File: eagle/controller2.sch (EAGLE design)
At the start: 15 parts, among them K1 SRD-05VDC-SL-C, K2 SRD-05VDC-SL-C, T1 BC547, T2 BC547, X1 VCC, X2 IN1, X3 IN2

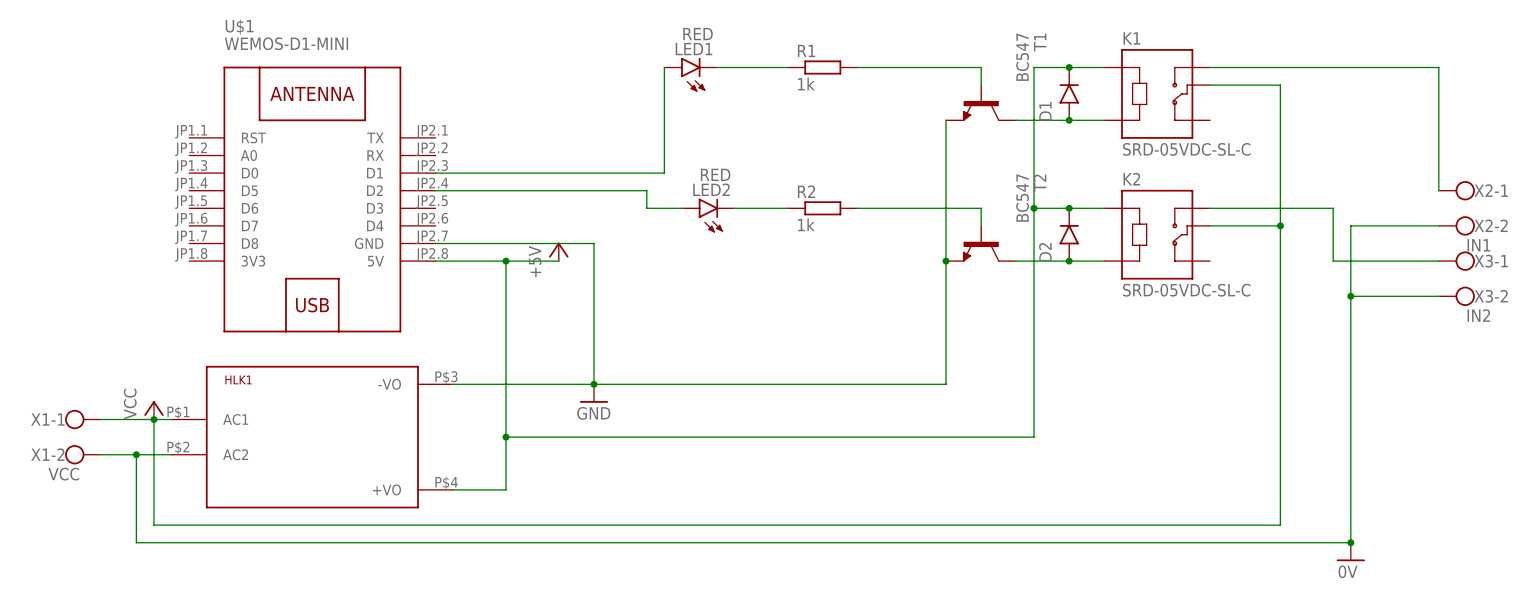
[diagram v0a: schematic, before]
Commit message: refactoring
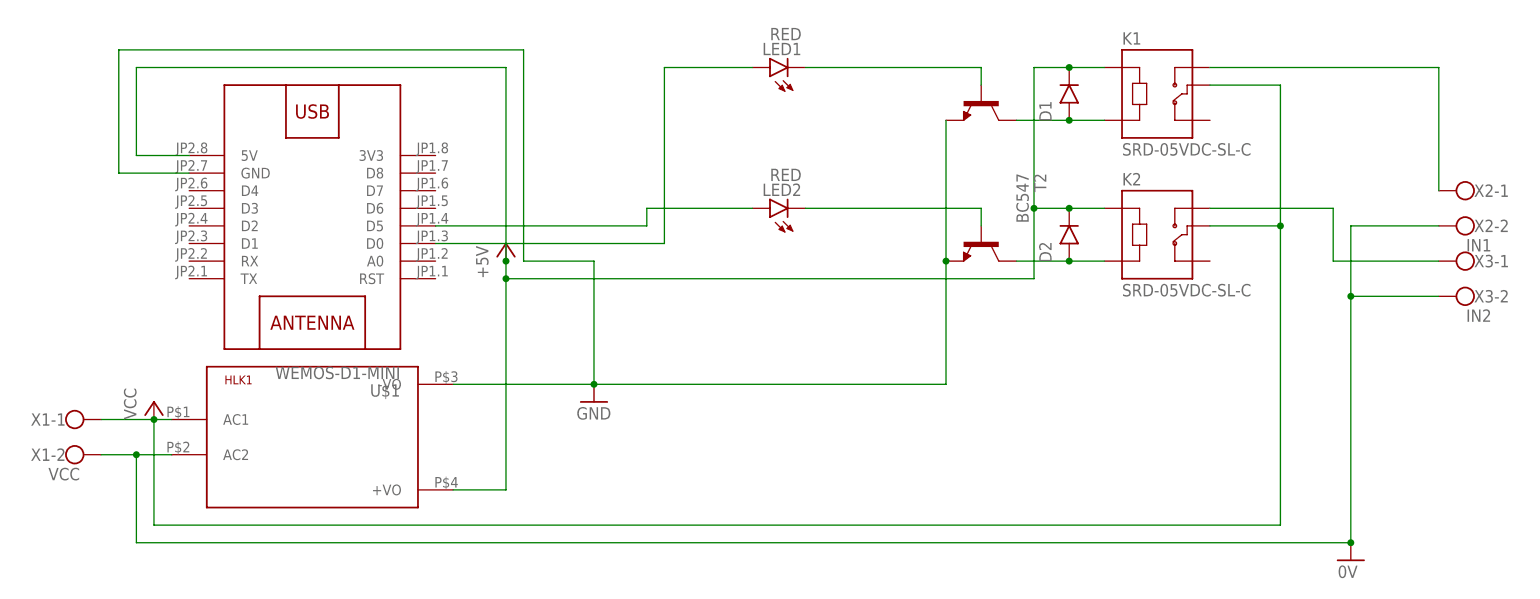
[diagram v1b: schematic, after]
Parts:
- removed R1, R2: 1k, rcl:R-EU_0204/5
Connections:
- removed net N$19: LED2.C, R2.1
- removed net N$20: LED1.C, R1.1
- net N$14: now also U$1.D5; no longer U$1.D2
- net N$15: now also U$1.D0; no longer U$1.D1
- net N$8: now also LED2.C; no longer R2.2
- net N$9: now also LED1.C; no longer R1.2
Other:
- moved on the sheet: LED1, LED2, U$1
